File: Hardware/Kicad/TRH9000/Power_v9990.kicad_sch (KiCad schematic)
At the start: 21 parts, among them U1 74HC138, U2 74HC32, U3 V9990, U4 KM428C256, U5 KM428C256, U6 LMH1980

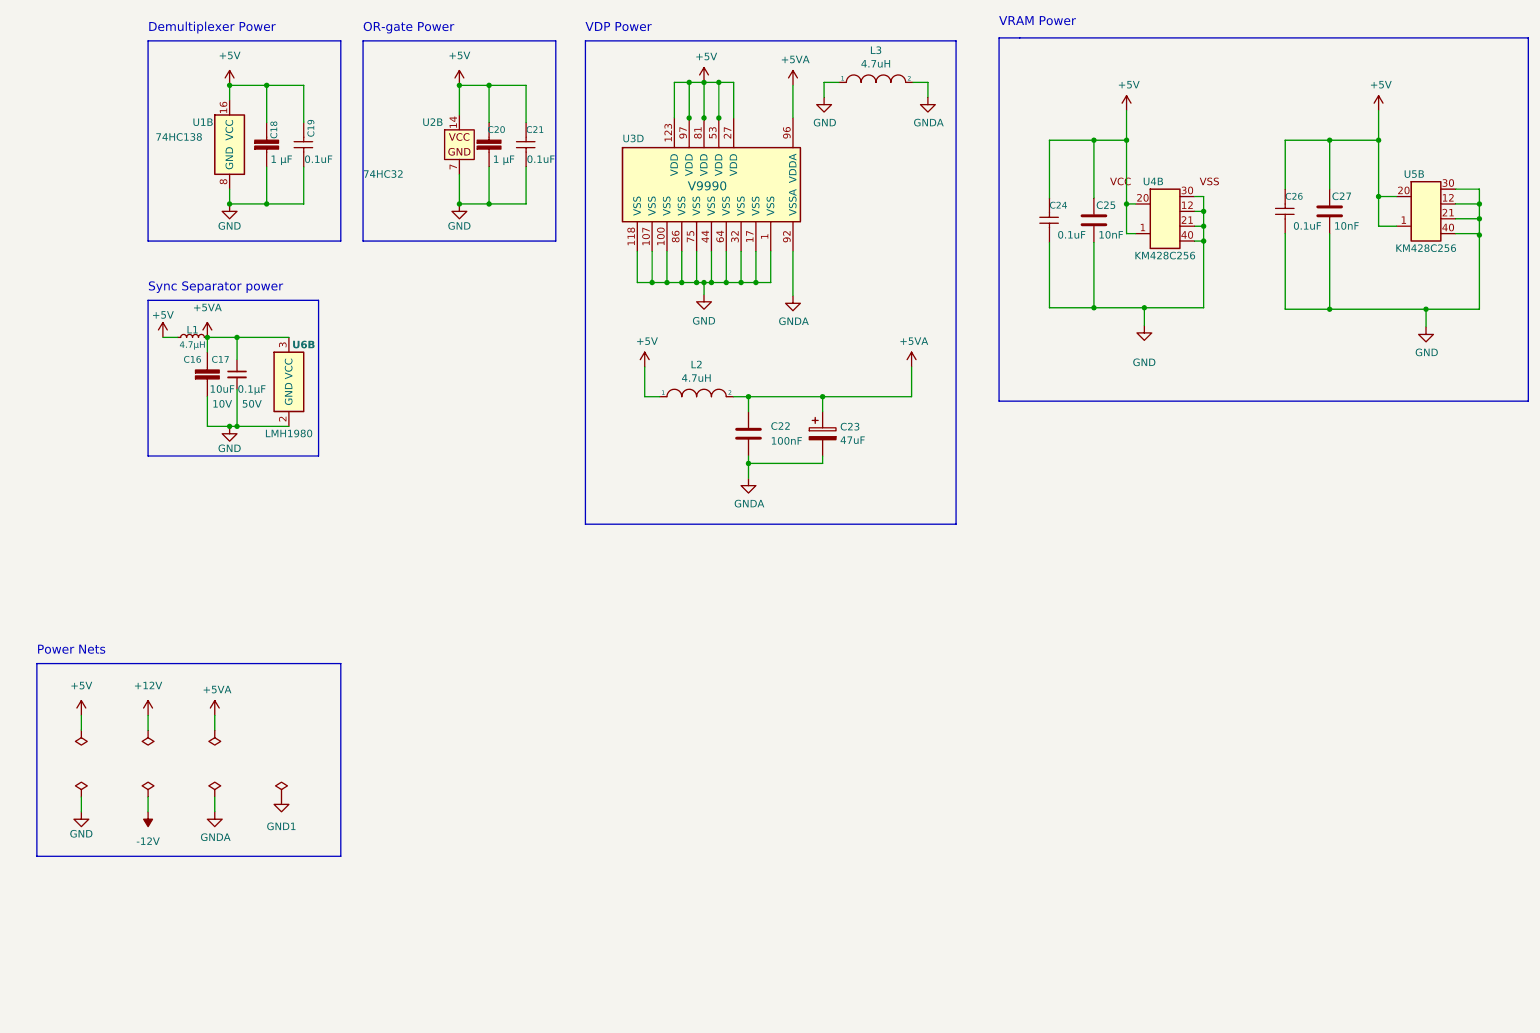
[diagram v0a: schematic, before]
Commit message: Multiple changes.
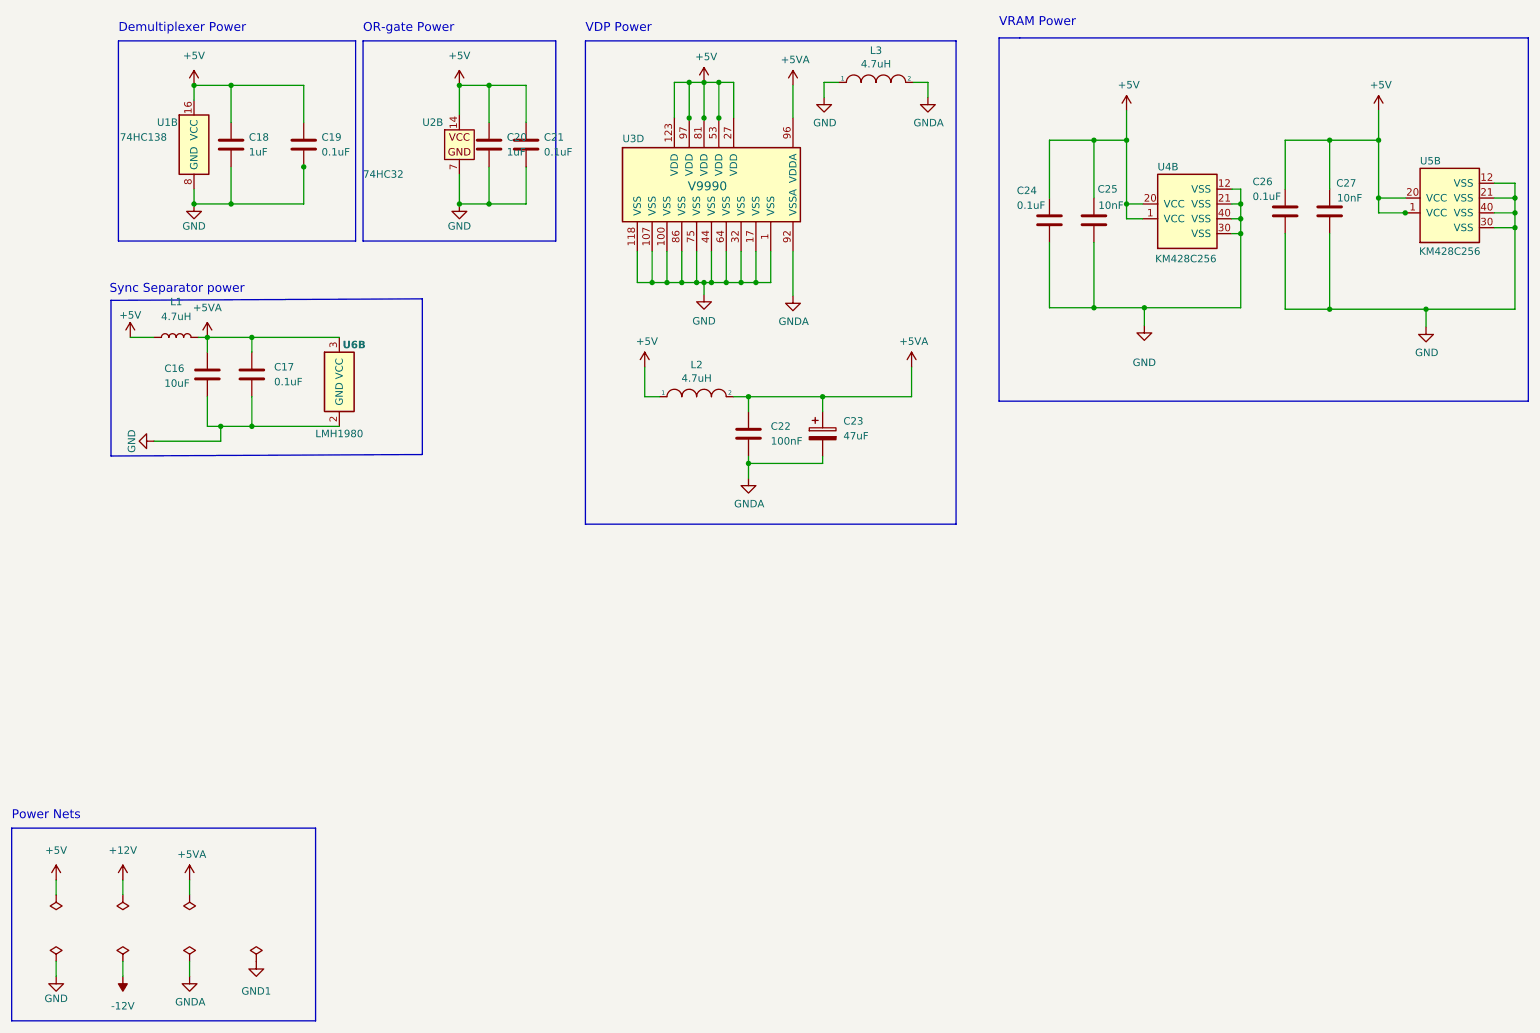
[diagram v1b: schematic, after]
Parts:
- removed C16: 10uF, Capacitor_SMD:C_0805_2012Metric, symbol LRJ-parts:C_GRM21BR71A106KA73K
- removed C17: 0.1µF, Capacitor_SMD:C_0805_2012Metric, symbol LRJ-parts:C_CL10B104KB8NNNL
- removed C18, C20: 1 µF, Capacitor_SMD:C_0805_2012Metric, symbol LRJ-parts:C_CL21B105KBFNNNF
- removed C19, C21, C24, C26: 0.1uF, Capacitor_SMD:C_0805_2012Metric, symbol LRJ-parts:C_CC0805JPX7R9BB104
- removed C23: 47uF, Capacitor_THT:CP_Radial_D5.0mm_P2.50mm, symbol Device:CP
- removed L1: 4.7µH, Inductor_SMD:L_1206_3216Metric, symbol LRJ-parts:L_MLZ2012M4R7HT000
- added C16: 10uF, Capacitor_SMD:C_0805_2012Metric, symbol Device:C
- added C17, C19, C21, C24, C26: 0.1uF, Capacitor_SMD:C_0805_2012Metric, symbol Device:C
- added C18, C20: 1uF, Capacitor_SMD:C_0805_2012Metric, symbol Device:C
- added C23: 47uF, Capacitor_Tantalum_SMD:CP_EIA-3528-15_AVX-H, symbol Device:C_Polarized
- added L1: 4.7uH, Inductor_SMD:L_0805_2012Metric, symbol Device:L
- L2, L3: footprint Inductor_SMD:L_1206_3216Metric -> Inductor_SMD:L_0805_2012Metric
- U6: symbol LRJ-parts:LMH1980 -> TRH9000:LMH1980
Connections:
- net +5V: now also C18.1, C19.1, C20.1, C21.1, C24.1, C26.1, L1.1
- net +5VA: now also C16.2, C17.1, C23.1, L1.2
- net GND: now also C16.1, C17.2, C18.2, C19.2, C20.2, C21.2, C24.2, C26.2
- net GNDA: now also C23.2
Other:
- moved on the sheet: U1B, U6B
